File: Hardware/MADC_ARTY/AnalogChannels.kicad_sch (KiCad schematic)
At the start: 37 parts, among them Q1 MMBT6429, Q10 MMBF4392, Q11 MMBT6429, Q12 MMBT6429, Q2 JFE2140D, Q3 MMBT6429, Q4 MMBF4392, Q5 MMBT6429, Q6 MMBT6429, Q7 MMBT6429, Q8 JFE2140D, Q9 MMBT6429, U1 OPA2192, U2 OPA4192IPW, U3 OPA4192IPW

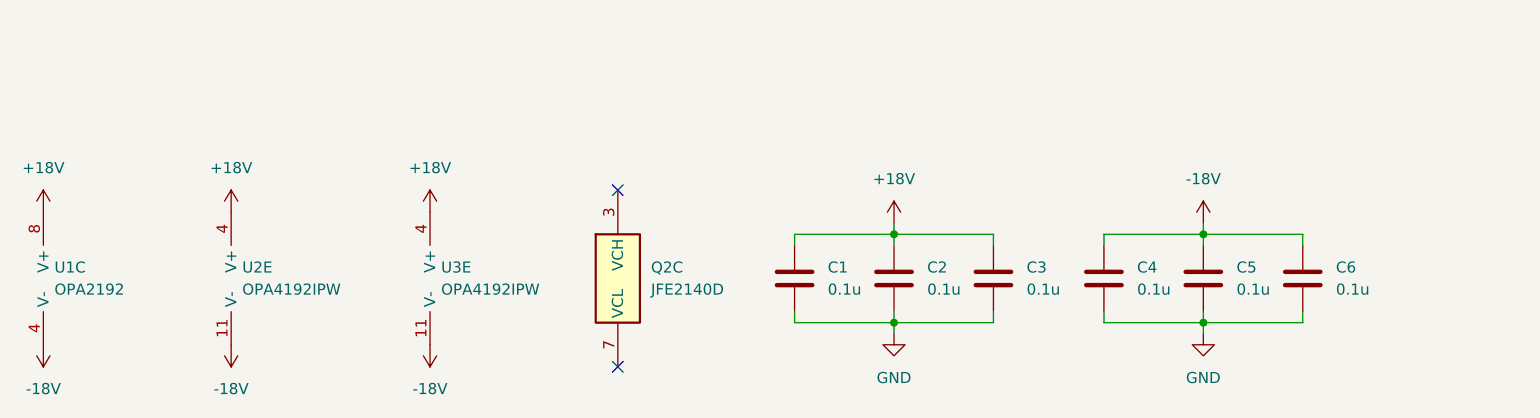
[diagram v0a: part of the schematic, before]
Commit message: Schematic
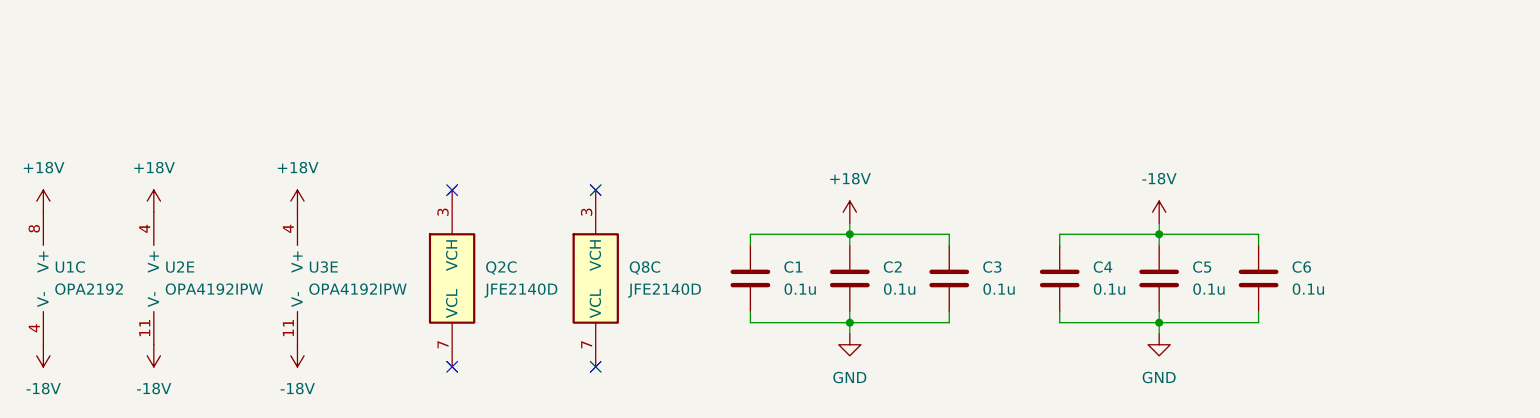
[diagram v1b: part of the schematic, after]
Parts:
- added unit 3 of Q8
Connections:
- no-connect marks 2 -> 4
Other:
- moved on the sheet: C1, C2, C3, C4, C5, C6, Q2C, U2E, U3E
